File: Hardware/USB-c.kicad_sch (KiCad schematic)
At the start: 9 parts, among them J1 USB4105-GF-A-120, U4 TPD2EUSB30DRTR

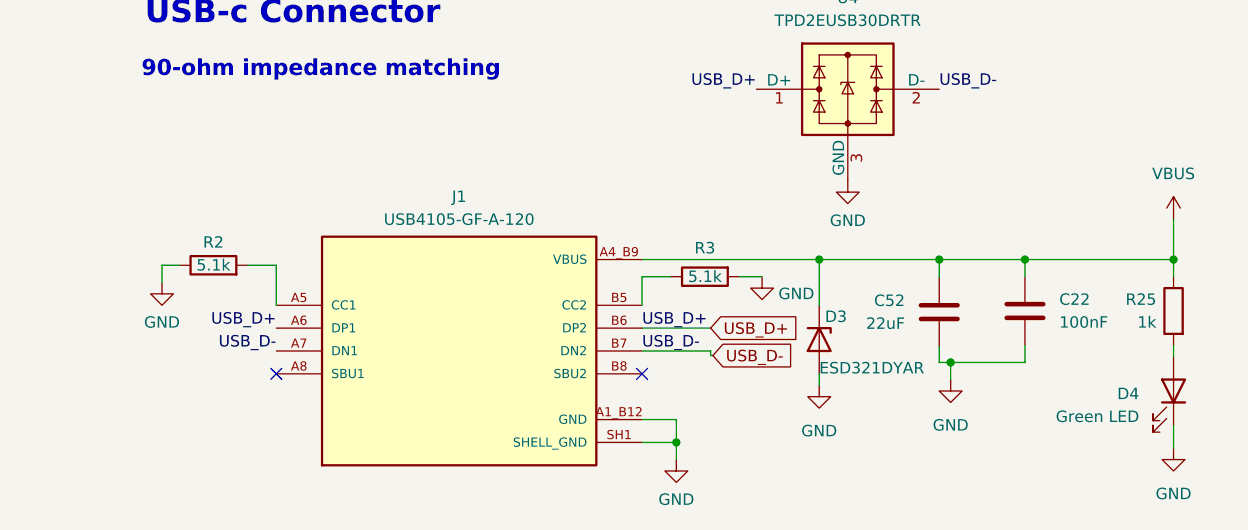
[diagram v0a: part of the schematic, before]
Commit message: Changed footprints, generated BOM
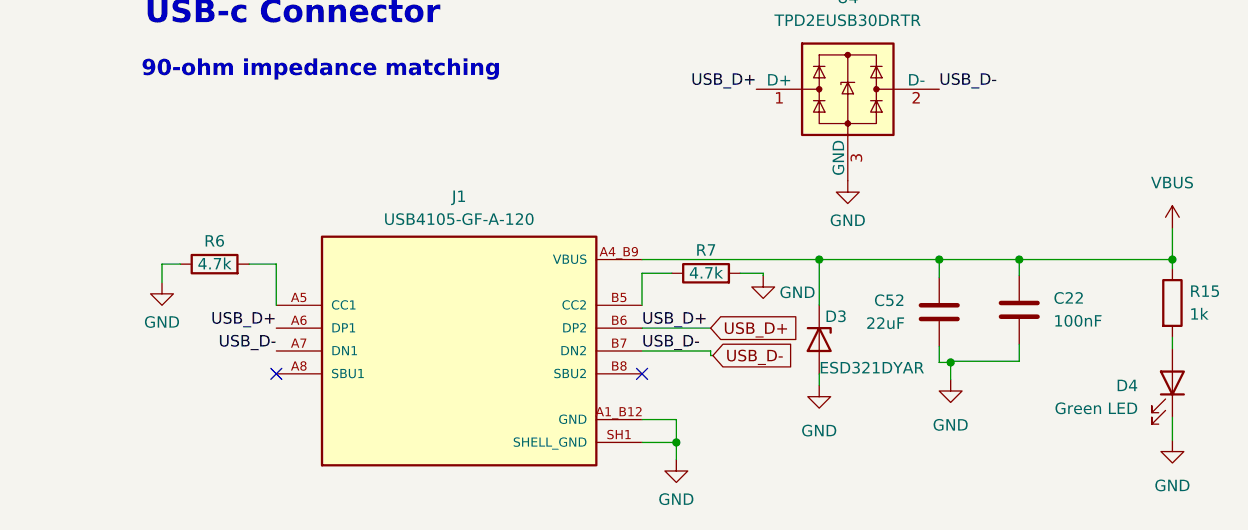
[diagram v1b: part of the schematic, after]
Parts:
- removed R2, R3: 5.1k, Resistor_SMD:R_0402_1005Metric, symbol Device:R
- removed R25: 1k, Resistor_SMD:R_0402_1005Metric, symbol Device:R
- added R15: 1k, Resistor_SMD:R_0603_1608Metric, symbol Device:R
- added R6, R7: 4.7k, Resistor_SMD:R_0603_1608Metric, symbol Device:R
- C22: footprint Capacitor_SMD:C_0402_1005Metric -> Capacitor_SMD:C_0603_1608Metric; Distributer Link https://www.ozdisan.com/p/smt-smd-ve-mlcc-kapasitorler-184/murata-grt155r71e104ke01d-1074547 -> https://www.ozdisan.com/p/smt-smd-ve-mlcc-kapasitorler-184/samsung-cl10b104ko8wpnc-522227; Part Number GRT155R71E104KE01D -> CL10B104KO8WPNC
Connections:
- net GND: now also R6.1, R7.2
- net VBUS: now also R15.1
- net at D4.2 (A): now also R15.2
- net at J1.A5 (CC1): now also R6.2
- net at J1.B5 (CC2): now also R7.1
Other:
- moved on the sheet: D4
